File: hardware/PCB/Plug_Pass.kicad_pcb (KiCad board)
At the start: 2 copper layers, 139.7 x 108 mm, 9 parts, among them J1 Conn_01x06, J10 TDPT-1017503, J2 Conn_01x08, J3 Conn_02x04_Odd_Even, J4 Conn_02x04_Odd_Even

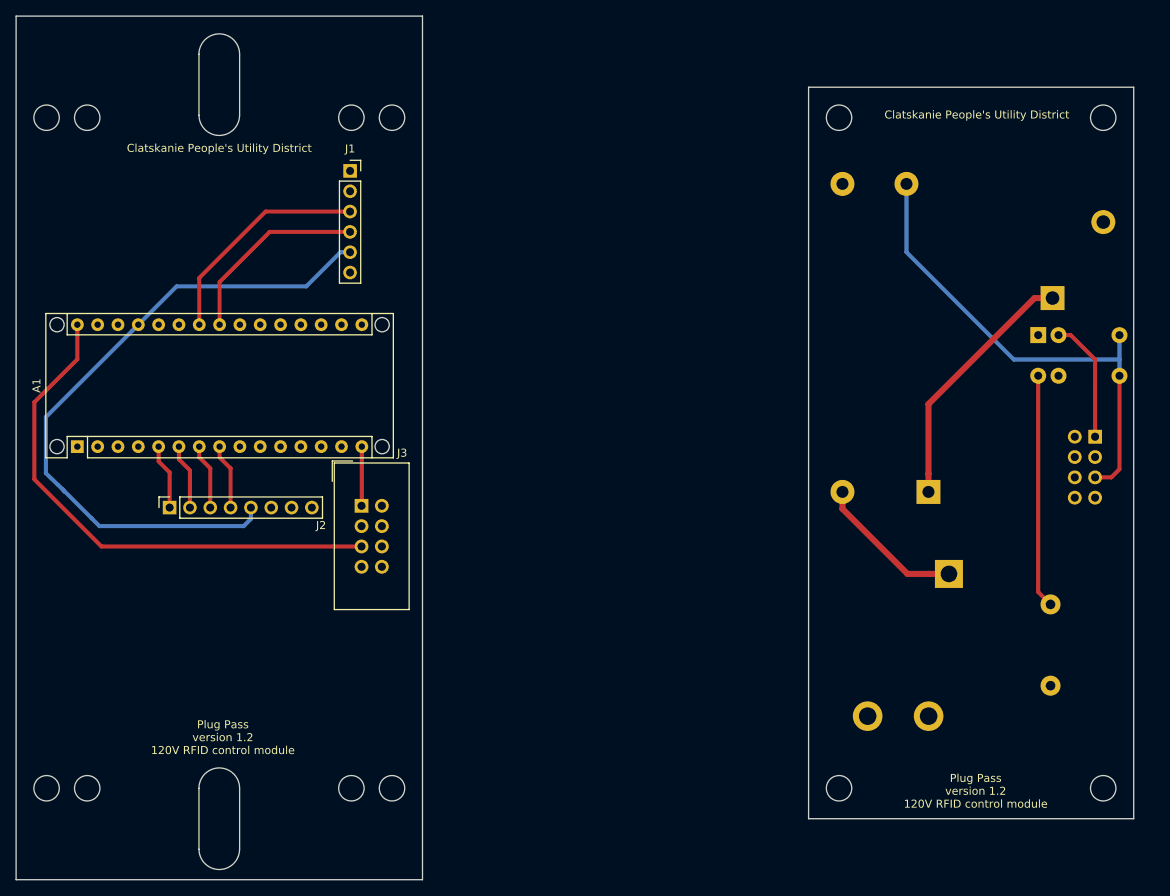
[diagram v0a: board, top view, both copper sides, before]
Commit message: Add files via upload
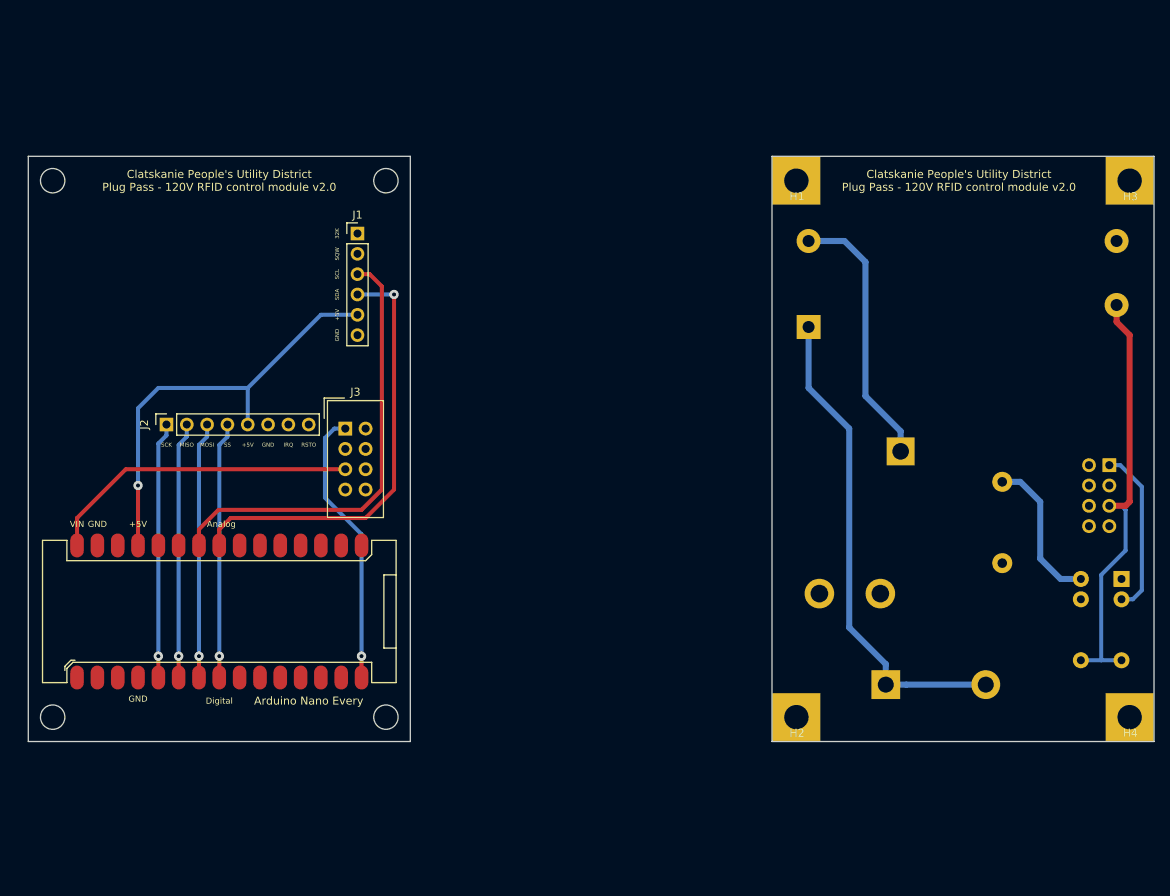
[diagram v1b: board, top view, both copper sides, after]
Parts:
- removed J10: TDPT-1017503, Plug_Pass:TDPT_2P_6.35MM
- added H1: MountingHole_Pad, Plug_Pass:Ground_Pad, F.Cu at (176.3, 62.5)
- added H2: MountingHole_Pad, Plug_Pass:Ground_Pad, F.Cu at (176.3, 129.5)
- added H3: MountingHole_Pad, Plug_Pass:Ground_Pad, F.Cu at (217.9, 62.5)
- added H4: MountingHole_Pad, Plug_Pass:Ground_Pad, F.Cu at (217.9, 129.5)
- added J6: Screw_Terminal_01x01, Plug_Pass:PLH5-1_75, B.Cu at (187.5, 125.5)
- A1: value Arduino_Nano_v3.x -> Arduino_Nano_Every; footprint Plug_Pass:Arduino_Nano_WithMountingHoles -> Plug_Pass:NANO_33_Footprint_SMD_Castell
- J1: footprint Plug_Pass:PinSocket_1x06_P2.54mm_Vertical -> Plug_Pass:RTC_PinHeader
- J2: footprint Plug_Pass:PinSocket_1x08_P2.54mm_Vertical -> Plug_Pass:PN532_NFC_PinSocket
- J3: footprint Plug_Pass:IDC-Header_2x04_P2.54mm_Vertical -> Plug_Pass:IDC-Header_2x04_P2.54mm_Vertical_Small
- moved RLY2 32.2 mm to (216.9, 112.3), turned to 270 degrees
- moved A1 27.2 mm to (104.1, 116.3), turned to 0 degrees
- moved PS1 25.5 mm to (177.8, 80.8), turned to 0 degrees
- moved RLY1 16.5 mm to (175.8, 93.0)
- moved J2 10.4 mm to (97.5, 93.0)
- moved J3 9.86 mm to (119.9, 93.5)
- moved J1 7.88 mm to (121.4, 69.1)
- moved J4 3.98 mm to (215.4, 98.0)
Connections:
- J3 pad 2: Net-(J3-Pad2) -> GNDREF
- J3 pad 4: Net-(J3-Pad4) -> GNDREF
- J3 pad 6: Net-(J3-Pad6) -> GNDREF
- J3 pad 8: Net-(J3-Pad8) -> GNDREF
- J4 pad 2: Net-(J4-Pad2) -> GNDREF
- J4 pad 4: Net-(J4-Pad4) -> GNDREF
- J4 pad 6: Net-(J4-Pad6) -> GNDREF
- J4 pad 8: Net-(J4-Pad8) -> GNDREF
- PS1 pad 1: Net-(J10-Pad1) -> NEUT
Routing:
- net NEUT: track 0.00 -> 61.2 mm
- net /RLY2-Pin: track 22.9 -> 56.0 mm, vias 0 -> 1
- net VCC: track 126.9 -> 94.9 mm
- net Net-(J10-Pad1): track 32.0 -> 0.00 mm
- net /SDA: track 24.2 -> 54.9 mm, vias 0 -> 1
- net +5V: track 84.1 -> 54.0 mm, vias 0 -> 1
- net /SCL: track 28.1 -> 56.0 mm
- net /SS: track 8.19 -> 32.0 mm, vias 0 -> 1
- net /SCK: track 8.19 -> 32.0 mm, vias 0 -> 1
- net /MOSI: track 8.19 -> 32.0 mm, vias 0 -> 1
- net /MISO: track 8.19 -> 32.0 mm, vias 0 -> 1
- net Net-(J9-Pad~): track 18.8 -> 33.7 mm
- net /RLY1-Pin: track 29.2 -> 19.0 mm
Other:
- board size 139.7 x 108 mm -> 140.7 x 73.2 mm
- board text added: "Clatskanie People's Utility District Plug Pass - 120V RFID control module v2.0"
- board text added: "Clatskanie People's Utility District Plug Pass - v2.0 - AC shield"
- board text added: "Clatskanie People's Utility District Plug Pass - v2.0 - arduino shield"
- board text added: "GND"
- board text removed: "Clatskanie People's Utility District"
- board text removed: "Plug Pass version 1.2 120V RFID control module"
- board text removed: "Plug Pass version 1.2 AC shield"
- board text removed: "Plug Pass version 1.2 arduino shield"
